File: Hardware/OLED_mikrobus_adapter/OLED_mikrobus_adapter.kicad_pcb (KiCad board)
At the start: 2 copper layers, 28 x 38.8 mm, 9 parts, among them J1 Conn_01x08, J2 Conn_01x08, J3 Conn_01x04

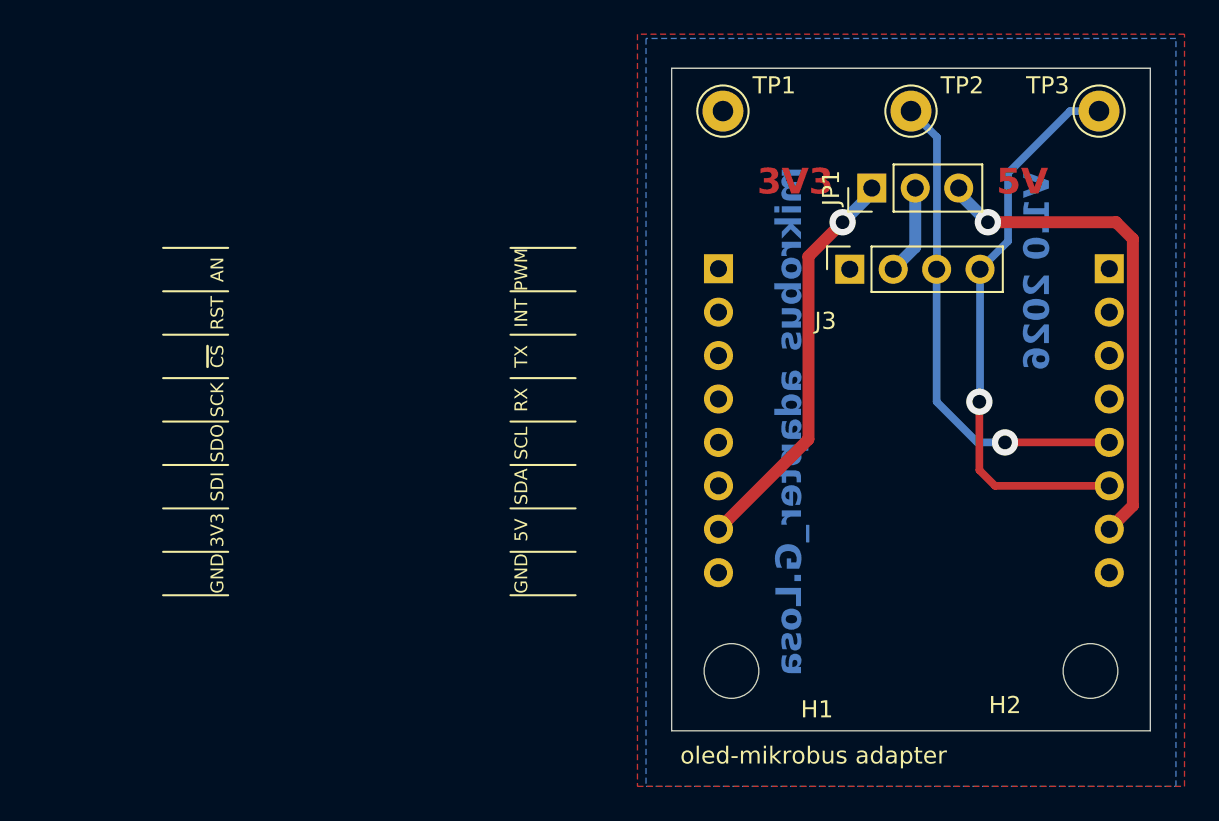
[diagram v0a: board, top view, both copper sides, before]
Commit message: improved PCB layout
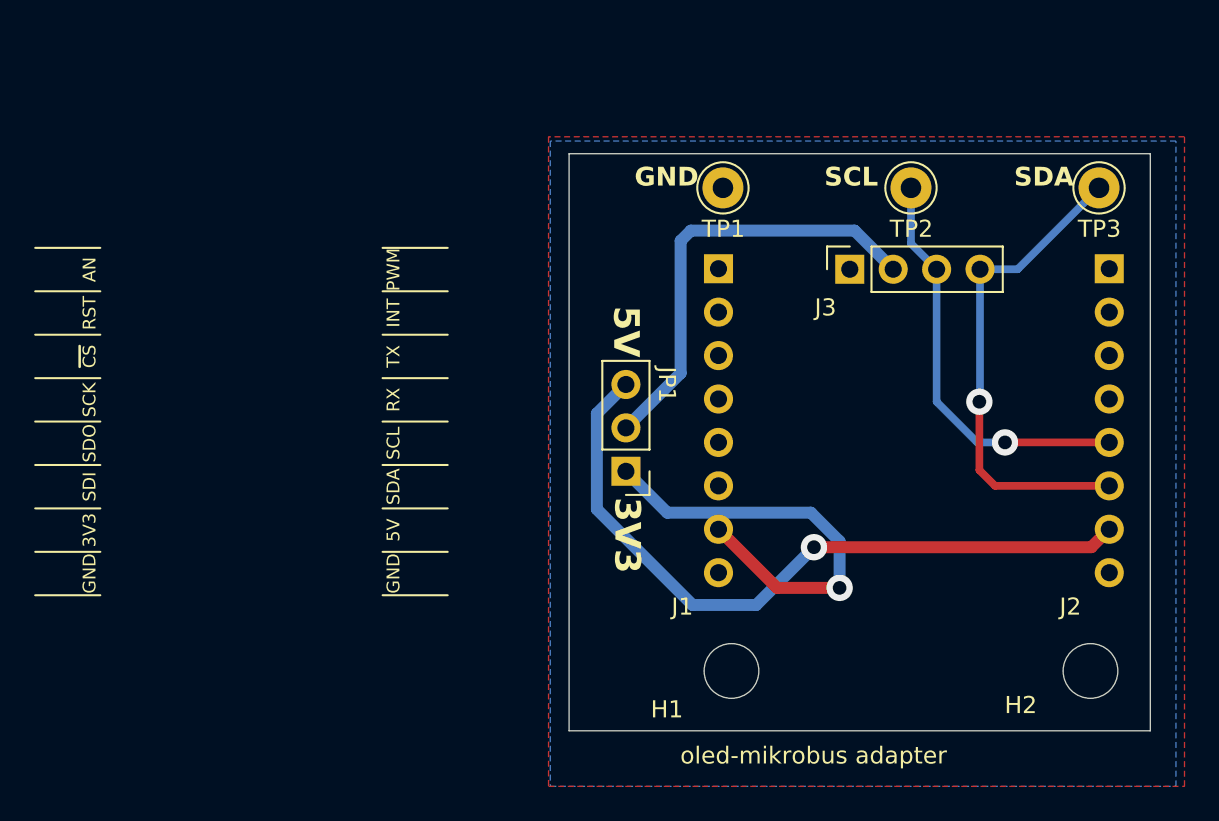
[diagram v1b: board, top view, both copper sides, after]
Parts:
- moved JP1 21.9 mm to (67.3, 65.6), turned to 180 degrees
- moved TP1 4.49 mm to (73.0, 49.0)
- moved TP2 4.49 mm to (84.0, 49.0)
- moved TP3 4.49 mm to (95.0, 49.0)
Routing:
- net /VDD: track 5.28 -> 25.9 mm
- net +5V: track 29.4 -> 42.1 mm
- net /SCL: track 28.7 -> 24.2 mm
- net /SDA: track 32.9 -> 28.7 mm
- net +3V3: track 23.9 -> 25.4 mm
- added copper zone on F.Cu, net GND
- removed copper zone on F.Cu, net (none)
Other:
- board size 28 x 38.8 mm -> 34 x 33.8 mm
- board text added: "OLED-µBUS-adapter"
- board text added: "V1.0-2026-G.Losa"
- board text removed: "V1.0 2026"
- board text removed: "mikrobus_adapter_G.Losa"
